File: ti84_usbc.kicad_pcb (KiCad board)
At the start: 2 copper layers, 10.2 x 10.9 mm, 6 parts, among them J1 USB_C_Receptacle_USB2.0, J2 USB_OTG, U1 TUSB320

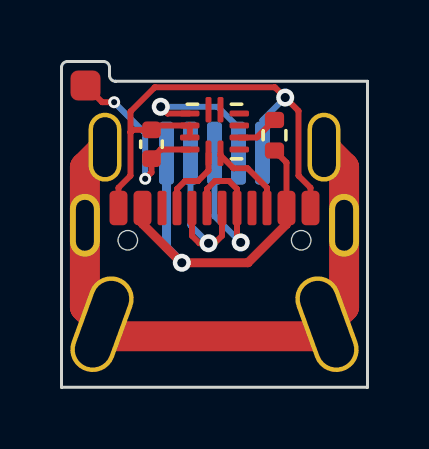
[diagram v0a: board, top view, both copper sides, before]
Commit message: Add files via upload
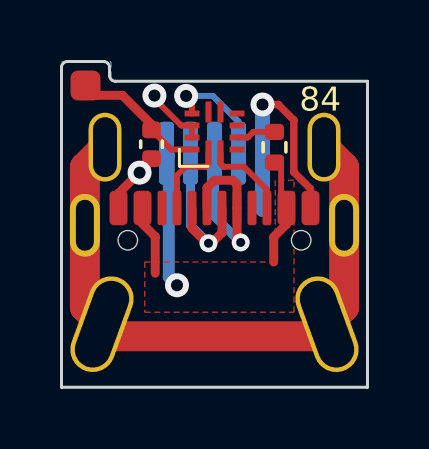
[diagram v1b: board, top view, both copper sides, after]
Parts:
- U1: footprint Package_DFN_QFN:Texas_X2QFN-12_1.6x1.6mm_P0.4mm -> ti84_mini_usb:IC_TUSB320IRWBR
- moved R1 0.40 mm to (190.0, 28.4)
- turned C1 to 90 degrees
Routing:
- net GND: track 17.7 -> 12.2 mm, vias 1 -> 3
- net /VBUS: track 13.0 -> 10.6 mm
- net +BATT: track 6.33 -> 4.54 mm, vias 2 -> 0
- net /ID: track 4.79 -> 3.82 mm
- added copper zone on F.Cu, net /VBUS
- added copper zone on B.Cu, net GND
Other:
- board text added: "84"
